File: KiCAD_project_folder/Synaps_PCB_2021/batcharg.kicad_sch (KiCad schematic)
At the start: 26 parts, among them U6 MP2615GQ-Z, U7 BQ771808DPJR

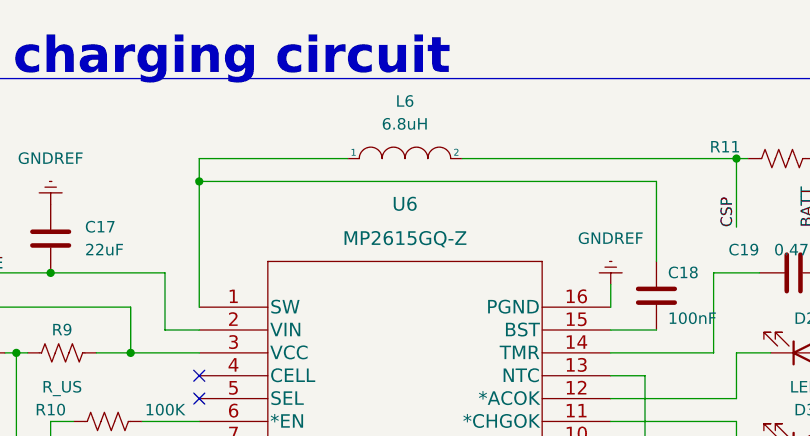
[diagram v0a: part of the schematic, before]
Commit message: schematic finished
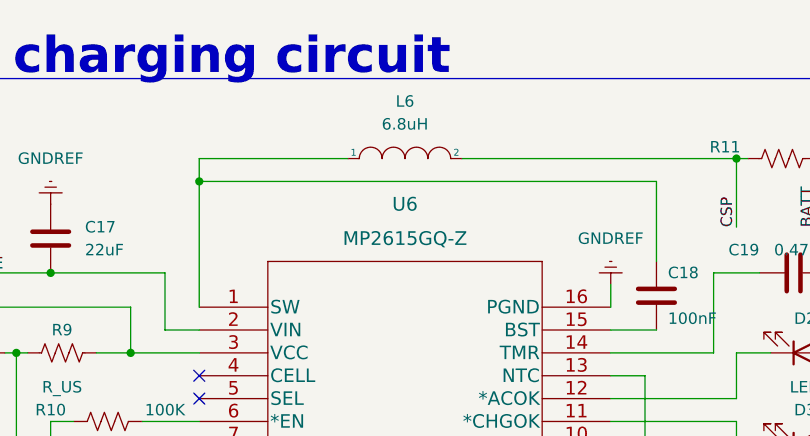
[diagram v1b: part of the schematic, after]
